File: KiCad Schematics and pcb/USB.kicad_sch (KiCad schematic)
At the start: 16 parts, among them IC4 TPS25730DREFR, J7 USB_C_Receptacle_USB2.0_16P, U1 TVS2200DRV

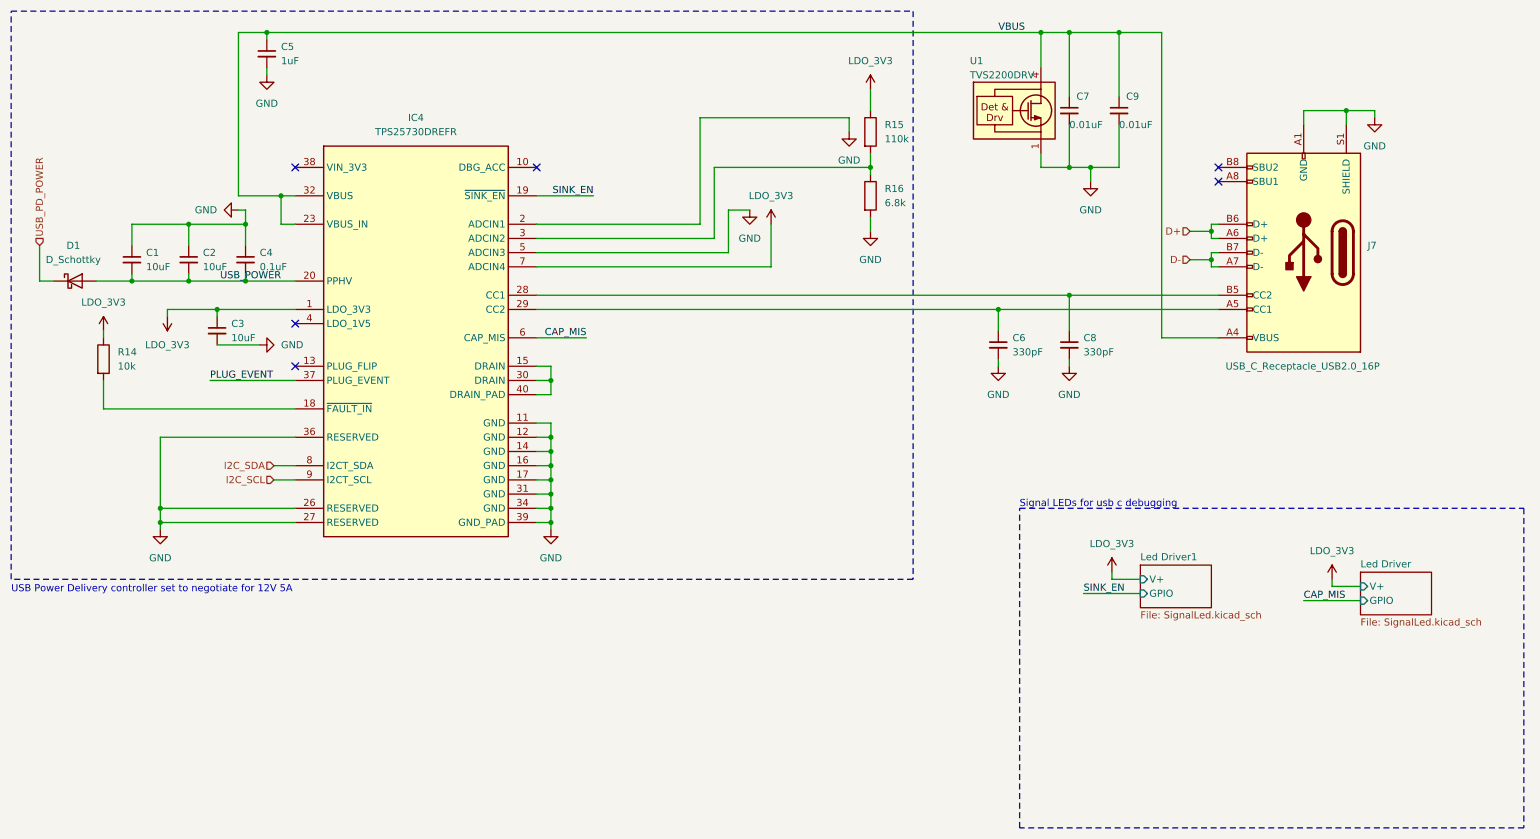
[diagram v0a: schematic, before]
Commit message: v0.1
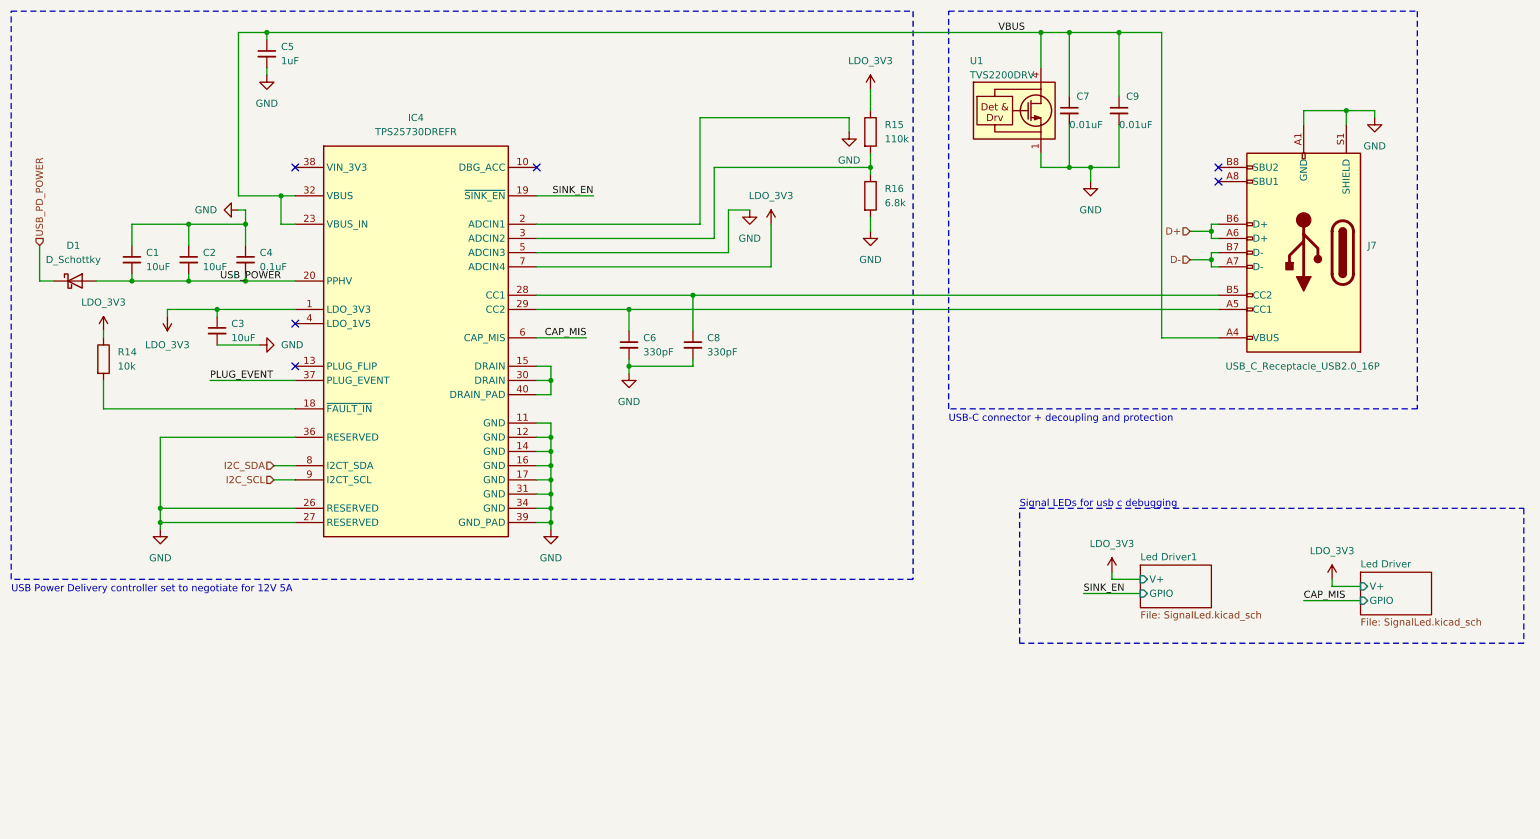
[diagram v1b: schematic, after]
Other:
- note added: "USB-C connector + decoupling and protection"
- moved on the sheet: C6, C8
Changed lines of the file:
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@@
   (junction (at 49.53 66.04) (diameter 0) (color 0 0 0 0)
   )
+  (junction (at 123.19 76.2) (diameter 0) (color 0 0 0 0)
+  )
   (junction (at 109.22 104.14) (diameter 0) (color 0 0 0 0)
   )
@@
   (junction (at 34.29 60.96) (diameter 0) (color 0 0 0 0)
   )
+  (junction (at 123.19 66.04) (diameter 0) (color 0 0 0 0)
+  )
   (junction (at 44.45 60.96) (diameter 0) (color 0 0 0 0)
   )
@@
   (junction (at 210.82 16.51) (diameter 0) (color 0 0 0 0)
   )
-  (junction (at 189.23 66.04) (diameter 0) (color 0 0 0 0)
-  )
-  (junction (at 201.93 63.5) (diameter 0) (color 0 0 0 0)
-  )
   (junction (at 227.33 52.07) (diameter 0) (color 0 0 0 0)
   )
@@
   )
   (junction (at 251.46 30.48) (diameter 0) (color 0 0 0 0)
+  )
+  (junction (at 134.62 63.5) (diameter 0) (color 0 0 0 0)
   )
   (junction (at 205.74 40.64) (diameter 0) (color 0 0 0 0)
@@
     (stroke (width 0) (type default))
   )
-  (wire (pts (xy 201.93 63.5) (xy 228.6 63.5))
+  (wire (pts (xy 134.62 63.5) (xy 228.6 63.5))
     (stroke (width 0) (type default))
   )
@@
     (stroke (width 0) (type default))
   )
-  (wire (pts (xy 189.23 66.04) (xy 228.6 66.04))
+  (wire (pts (xy 123.19 66.04) (xy 228.6 66.04))
     (stroke (width 0) (type default))
   )
@@
     (stroke (width 0) (type default))
   )
-  (wire (pts (xy 201.93 63.5) (xy 201.93 69.85))
+  (wire (pts (xy 134.62 63.5) (xy 134.62 69.85))
     (stroke (width 0) (type default))
   )
@@
     (stroke (width 0) (type default))
   )
-  (wire (pts (xy 189.23 66.04) (xy 189.23 69.85))
+  (wire (pts (xy 123.19 66.04) (xy 123.19 69.85))
     (stroke (width 0) (type default))
   )
@@
     (stroke (width 0) (type default))
   )
-  (wire (pts (xy 106.68 63.5) (xy 201.93 63.5))
+  (wire (pts (xy 106.68 63.5) (xy 134.62 63.5))
     (stroke (width 0) (type default))
   )
@@
     (stroke (width 0) (type default))
   )
+  (wire (pts (xy 123.19 76.2) (xy 134.62 76.2))
+    (stroke (width 0) (type default))
+  )
   (wire (pts (xy 135.89 50.8) (xy 106.68 50.8))
     (stroke (width 0) (type default))
@@
     (stroke (width 0) (type default))
   )
-  (wire (pts (xy 201.93 74.93) (xy 201.93 76.2))
+  (wire (pts (xy 134.62 74.93) (xy 134.62 76.2))
     (stroke (width 0) (type default))
   )
@@
     (stroke (width 0) (type default))
   )
-  (wire (pts (xy 189.23 74.93) (xy 189.23 76.2))
+  (wire (pts (xy 123.19 77.47) (xy 123.19 76.2))
+    (stroke (width 0) (type default))
+  )
+  (wire (pts (xy 123.19 74.93) (xy 123.19 76.2))
     (stroke (width 0) (type default))
   )
@@
     (stroke (width 0) (type default))
   )
-  (wire (pts (xy 106.68 66.04) (xy 189.23 66.04))
+  (wire (pts (xy 106.68 66.04) (xy 123.19 66.04))
     (stroke (width 0) (type default))
   )
@@
     (stroke (width 0) (type default))
   )
-  (rectangle (start 193.04 101.6) (end 283.21 158.75)
+  (rectangle (start 193.04 101.6) (end 283.21 125.73)
+    (stroke (width 0) (type dash))
+    (fill (type none))
+  )
+  (rectangle (start 180.34 12.7) (end 264.16 83.82)
     (stroke (width 0) (type dash))
     (fill (type none))
@@
     (stroke (width 0) (type dash))
     (fill (type none))
+  )
+  (text "USB-C connector + decoupling and protection" (at 180.34 86.36 0)
+    (effects (font (size 1.27 1.27)) (justify left bottom))
   )
   (text "Signal LEDs for usb c debugging" (at 193.04 101.6 0)
@@
     )
   )
-  (symbol (lib_id "power:GND") (at 189.23 76.2 0) (unit 1)
-    (in_bom yes) (on_board yes) (dnp no) (fields_autoplaced)
-    (property "Reference" "#PWR055" (at 189.23 82.55 0)
-      (effects (font (size 1.27 1.27)) hide)
-    )
-    (property "Value" "GND" (at 189.23 81.28 0)
-      (effects (font (size 1.27 1.27)))
-    )
-    (property "Footprint" "" (at 189.23 76.2 0)
-      (effects (font (size 1.27 1.27)) hide)
-    )
-    (property "Datasheet" "" (at 189.23 76.2 0)
+  (symbol (lib_id "power:GND") (at 123.19 77.47 0) (unit 1)
+    (in_bom yes) (on_board yes) (dnp no) (fields_autoplaced)
+    (property "Reference" "#PWR055" (at 123.19 83.82 0)
+      (effects (font (size 1.27 1.27)) hide)
+    )
+    (property "Value" "GND" (at 123.19 82.55 0)
+      (effects (font (size 1.27 1.27)))
+    )
+    (property "Footprint" "" (at 123.19 77.47 0)
+      (effects (font (size 1.27 1.27)) hide)
+    )
+    (property "Datasheet" "" (at 123.19 77.47 0)
       (effects (font (size 1.27 1.27)) hide)
     )
@@
     )
   )
-  (symbol (lib_id "Device:C_Small") (at 189.23 72.39 0) (unit 1)
-    (in_bom yes) (on_board yes) (dnp no) (fields_autoplaced)
-    (property "Reference" "C6" (at 191.77 71.1263 0)
-      (effects (font (size 1.27 1.27)) (justify left))
-    )
-    (property "Value" "330pF" (at 191.77 73.6663 0)
-      (effects (font (size 1.27 1.27)) (justify left))
-    )
-    (property "Footprint" "Capacitor_SMD:C_0805_2012Metric" (at 189.23 72.39 0)
-      (effects (font (size 1.27 1.27)) hide)
-    )
-    (property "Datasheet" "~" (at 189.23 72.39 0)
+  (symbol (lib_id "Device:C_Small") (at 123.19 72.39 0) (unit 1)
+    (in_bom yes) (on_board yes) (dnp no) (fields_autoplaced)
+    (property "Reference" "C6" (at 125.73 71.1263 0)
+      (effects (font (size 1.27 1.27)) (justify left))
+    )
+    (property "Value" "330pF" (at 125.73 73.6663 0)
+      (effects (font (size 1.27 1.27)) (justify left))
+    )
+    (property "Footprint" "Capacitor_SMD:C_0805_2012Metric" (at 123.19 72.39 0)
+      (effects (font (size 1.27 1.27)) hide)
+    )
+    (property "Datasheet" "~" (at 123.19 72.39 0)
       (effects (font (size 1.27 1.27)) hide)
     )
@@
         (path "/5cdf3b4f-d143-42e3-ac6f-eec5265de1fa/f403fb1f-6c3a-4b91-96f2-7610e89c4ca7"
           (reference "C7") (unit 1)
-        )
-      )
-    )
-  )
-  (symbol (lib_id "power:GND") (at 201.93 76.2 0) (unit 1)
-    (in_bom yes) (on_board yes) (dnp no) (fields_autoplaced)
-    (property "Reference" "#PWR056" (at 201.93 82.55 0)
-      (effects (font (size 1.27 1.27)) hide)
-    )
-    (property "Value" "GND" (at 201.93 81.28 0)
-      (effects (font (size 1.27 1.27)))
-    )
-    (property "Footprint" "" (at 201.93 76.2 0)
-      (effects (font (size 1.27 1.27)) hide)
-    )
-    (property "Datasheet" "" (at 201.93 76.2 0)
-      (effects (font (size 1.27 1.27)) hide)
-    )
-    (pin "1")
-    (instances
-      (project "ESPHome AIO"
-        (path "/5cdf3b4f-d143-42e3-ac6f-eec5265de1fa/f403fb1f-6c3a-4b91-96f2-7610e89c4ca7"
-          (reference "#PWR056") (unit 1)
         )
       )
@@
     )
   )
-  (symbol (lib_id "Device:C_Small") (at 201.93 72.39 0) (unit 1)
-    (in_bom yes) (on_board yes) (dnp no) (fields_autoplaced)
-    (property "Reference" "C8" (at 204.47 71.1263 0)
-      (effects (font (size 1.27 1.27)) (justify left))
-    )
-    (property "Value" "330pF" (at 204.47 73.6663 0)
-      (effects (font (size 1.27 1.27)) (justify left))
-    )
-    (property "Footprint" "Capacitor_SMD:C_0805_2012Metric" (at 201.93 72.39 0)
-      (effects (font (size 1.27 1.27)) hide)
-    )
-    (property "Datasheet" "~" (at 201.93 72.39 0)
-      (effects (font (size 1.27 1.27)) hide)
-    )
+  (symbol (lib_id "Device:C_Small") (at 134.62 72.39 0) (unit 1)
+    (in_bom yes) (on_board yes) (dnp no) (fields_autoplaced)
+    (property "Reference" "C8" (at 137.16 71.1263 0)
+      (effects (font (size 1.27 1.27)) (justify left))
+    )
+    (property "Value" "330pF" (at 137.16 73.6663 0)
+      (effects (font (size 1.27 1.27)) (justify left))
+    )
+    (property "Footprint" "Capacitor_SMD:C_0805_2012Metric" (at 134.62 72.39 0)
+      (effects (font (size 1.27 1.27)) hide)
+    )
+    (property "Datasheet" "~" (at 134.62 72.39 0)
+      (effects (font (size 1.27 1.27)) hide)
+    )
